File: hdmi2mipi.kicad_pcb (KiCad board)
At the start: 2 copper layers, 60.9 x 56.6 mm, 66 parts, among them J1 USB_C_Receptacle_USB2.0, J4 TP, J5 SWD, J6 BOOT, J7 SWD, Q1 BC846, Q2 BC846, Q3 BC846, Q4 BC846, Q5 BC846, Q6 BC846, U1 SY8079AAC, U3 SY6280AAC, U4 PCA9306DC, U6 W25Q16JVUXIQ, U8 SY6280AAC, X1 SG-210STF, Y1 12MHz

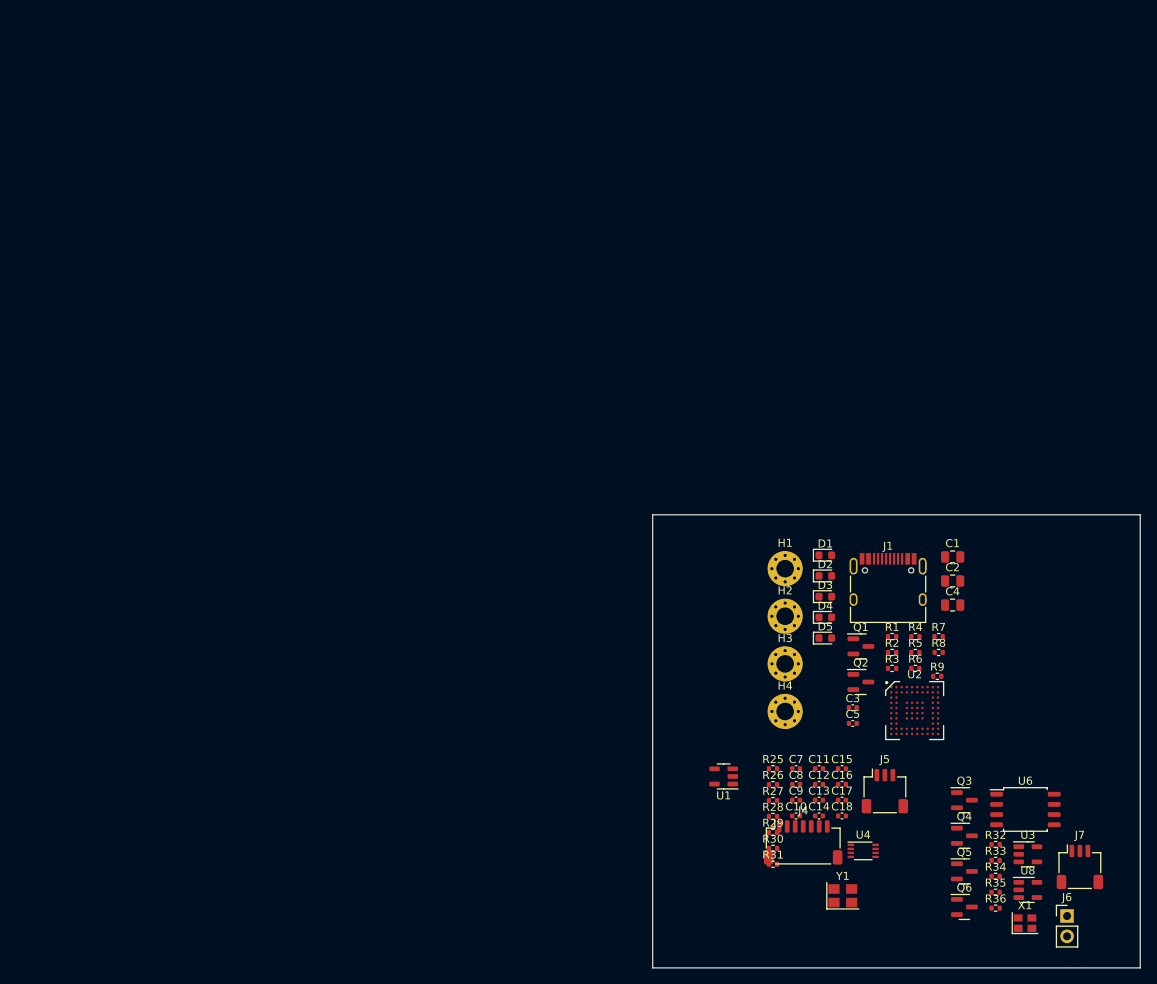
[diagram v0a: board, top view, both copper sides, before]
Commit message: Most of schematic done, experimenting with component placement
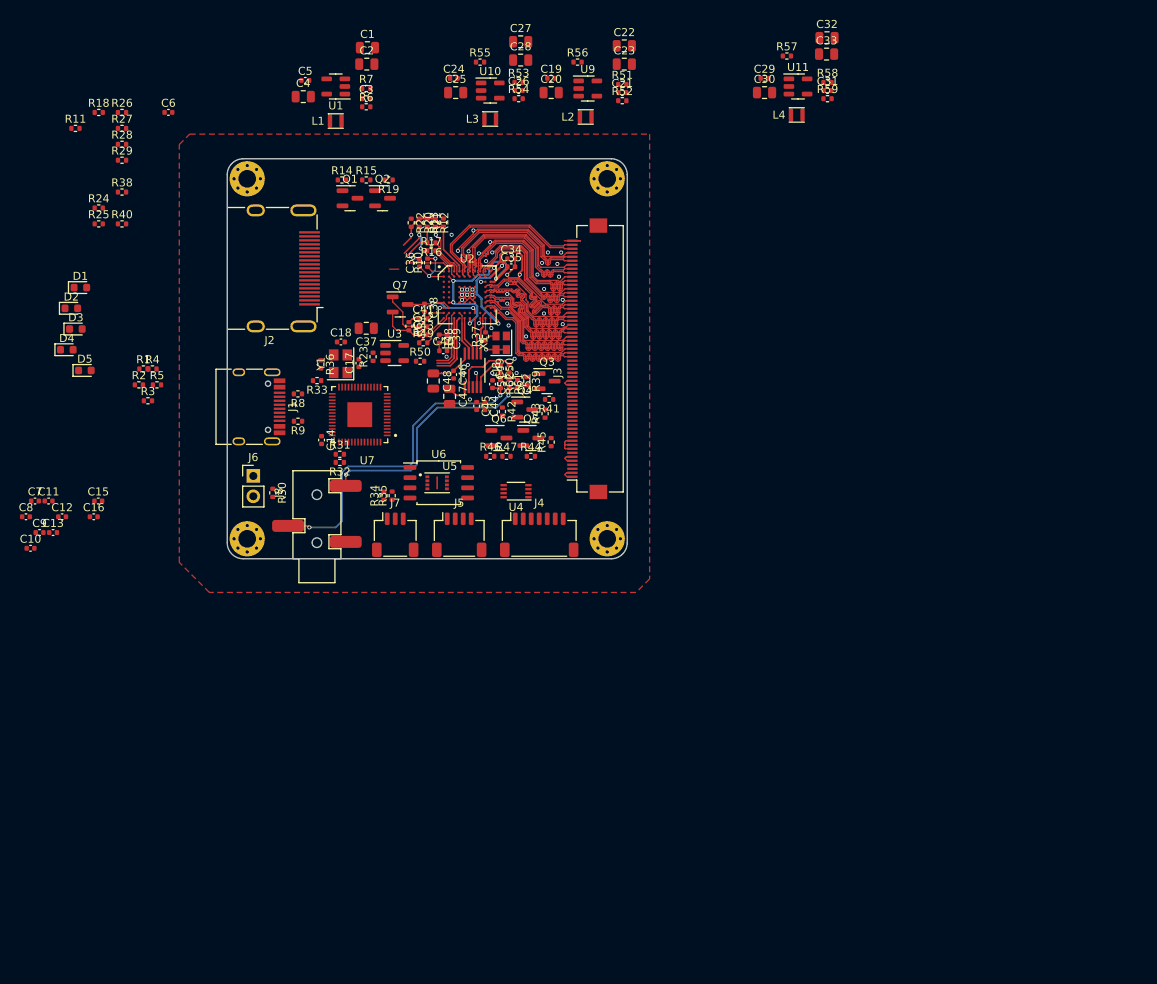
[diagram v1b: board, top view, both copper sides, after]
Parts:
- added C19: 100n, Capacitor_SMD:C_0402_1005Metric, F.Cu at (15.5, -35.1)
- added C20: 22u, Capacitor_SMD:C_0805_2012Metric, F.Cu at (15.5, -33.3)
- added C21: 22p, Capacitor_SMD:C_0402_1005Metric, F.Cu at (24.4, -33.3)
- added C22: 22u, Capacitor_SMD:C_0805_2012Metric, F.Cu at (24.6, -39.1)
- added C23: 22u, Capacitor_SMD:C_0805_2012Metric, F.Cu at (24.6, -36.8)
- added C24: 100n, Capacitor_SMD:C_0402_1005Metric, F.Cu at (3.33, -35.1)
- added C25: 22u, Capacitor_SMD:C_0805_2012Metric, F.Cu at (3.56, -33.3)
- added C26: 22p, Capacitor_SMD:C_0402_1005Metric, F.Cu at (11.4, -33.5)
- added C27: 22u, Capacitor_SMD:C_0805_2012Metric, F.Cu at (11.7, -39.6)
- added C28: 22u, Capacitor_SMD:C_0805_2012Metric, F.Cu at (11.7, -37.3)
- added C29: 100n, Capacitor_SMD:C_0402_1005Metric, F.Cu at (42.2, -35.1)
- added C30: 22u, Capacitor_SMD:C_0805_2012Metric, F.Cu at (42.2, -33.3)
- added C31: 22p, Capacitor_SMD:C_0402_1005Metric, F.Cu at (50.0, -33.5)
- added C32: 22u, Capacitor_SMD:C_0805_2012Metric, F.Cu at (50.0, -40.1)
- added C33: 22u, Capacitor_SMD:C_0805_2012Metric, F.Cu at (49.9, -38.1)
- added C34: 100n, Capacitor_SMD:C_0402_1005Metric, F.Cu at (10.5, -12.5)
- added C35: 100n, Capacitor_SMD:C_0402_1005Metric, F.Cu at (10.5, -11.5)
- added C36: 100n, Capacitor_SMD:C_0402_1005Metric, F.Cu at (-0.97, -12.0)
- added C37: 22u, Capacitor_SMD:C_0805_2012Metric, F.Cu at (-7.62, -3.81)
- added C38: 100n, Capacitor_SMD:C_0402_1005Metric, F.Cu at (-0.34, -6.39)
- added C39: 1n, Capacitor_SMD:C_0402_1005Metric, F.Cu at (2.50, -2.50)
- added C40: 0.1u, Capacitor_SMD:C_0402_1005Metric, F.Cu at (2.00, -1.00)
- added C41: 0.1u, Capacitor_SMD:C_0402_1005Metric, F.Cu at (-0.50, -5.00)
- added C42: 5p, Capacitor_SMD:C_0402_1005Metric, F.Cu at (-0.50, -4.00)
- added C43: 1n, Capacitor_SMD:C_0402_1005Metric, F.Cu at (-0.50, -3.00)
- added C44: 1u, Capacitor_SMD:C_0402_1005Metric, F.Cu at (7.21, 5.92)
- added C45: 100n, Capacitor_SMD:C_0402_1005Metric, F.Cu at (6.18, 5.90)
- added C46: 100n, Capacitor_SMD:C_0402_1005Metric, F.Cu at (3.30, 1.98)
- added C47: 47u, Capacitor_SMD:C_0805_2012Metric, F.Cu at (2.80, 4.70)
- added C48: 47u, Capacitor_SMD:C_0805_2012Metric, F.Cu at (0.76, 2.78)
- added C49: 100n, Capacitor_SMD:C_0402_1005Metric, F.Cu at (10.2, 1.24)
- added C50: 100n, Capacitor_SMD:C_0402_1005Metric, F.Cu at (9.15, 1.23)
- added C51: 39n, Capacitor_SMD:C_0402_1005Metric, F.Cu at (8.16, 3.17)
- added C52: 39n, Capacitor_SMD:C_0402_1005Metric, F.Cu at (11.3, 3.16)
- added C6: ~, Capacitor_SMD:C_0402_1005Metric, F.Cu at (-32.4, -30.8)
- added J2: HDMI_A_1.4, Connector_HDMI:HDMI_A_Molex_208658-1001_Horizontal, F.Cu at (-18.0, -11.3)
- added J3: ~, fpc60:Hirose_FH52-60S-0.5SH_1x60-1MP_P0.50mm_Horizontal, F.Cu at (20.0, 0.00)
- added J8: AudioJack3, custom:Boom-audiojack-PJ-320B, F.Cu at (-13.8, 21.0)
- added L1: 2.2u, custom:Inductor_MSC20FC, F.Cu at (-11.4, -29.7)
- added L2: 2.2u, custom:Inductor_MSC20FC, F.Cu at (19.8, -30.2)
- added L3: 2.2u, custom:Inductor_MSC20FC, F.Cu at (7.87, -30.0)
- added L4: 2.2u, custom:Inductor_MSC20FC, F.Cu at (46.2, -30.5)
- added Q7: 2SC2712, Package_TO_SOT_SMD:SOT-23, F.Cu at (-3.38, -6.79)
- added R10: 2k, Resistor_SMD:R_0402_1005Metric, F.Cu at (0.04, -12.0)
- added R11: 48k, Resistor_SMD:R_0402_1005Metric, F.Cu at (-44.0, -28.8)
- added R12: 0, Resistor_SMD:R_0402_1005Metric, F.Cu at (1.00, -17.0)
- added R13: 1.5k, Resistor_SMD:R_0402_1005Metric, F.Cu at (2.03, -17.0)
- added R14: 4.7k, Resistor_SMD:R_0402_1005Metric, F.Cu at (-10.7, -22.4)
- added R15: 10k, Resistor_SMD:R_0402_1005Metric, F.Cu at (-7.62, -22.4)
- added R16: 33, Resistor_SMD:R_0402_1005Metric, F.Cu at (0.52, -14.5)
- added R17: 33, Resistor_SMD:R_0402_1005Metric, F.Cu at (0.50, -13.5)
- added R18: 1k, Resistor_SMD:R_0402_1005Metric, F.Cu at (-41.1, -30.8)
- added R19: 1k, Resistor_SMD:R_0402_1005Metric, F.Cu at (-4.83, -22.4)
- added R20: 4.7k, Resistor_SMD:R_0402_1005Metric, F.Cu at (-1.00, -17.0)
- added R21: 4.7k, Resistor_SMD:R_0402_1005Metric, F.Cu at (0.00, -17.0)
- added R22: 100k, Resistor_SMD:R_0402_1005Metric, F.Cu at (-2.00, -17.0)
- added R23: 4.7k, Resistor_SMD:R_0402_1005Metric, F.Cu at (-6.77, -0.25)
- added R24: 4.7k, Resistor_SMD:R_0402_1005Metric, F.Cu at (-41.1, -18.9)
- added R37: 33, Resistor_SMD:R_0402_1005Metric, F.Cu at (7.29, -2.79)
- added R38: 10k, Resistor_SMD:R_0402_1005Metric, F.Cu at (-38.1, -20.8)
- added R39: 10k, Resistor_SMD:R_0402_1005Metric, F.Cu at (12.4, 2.79)
- added R40: 10k, Resistor_SMD:R_0402_1005Metric, F.Cu at (-38.1, -16.9)
- added R41: 4.7k, Resistor_SMD:R_0402_1005Metric, F.Cu at (15.2, 5.08)
- added R42: 10k, Resistor_SMD:R_0402_1005Metric, F.Cu at (9.40, 6.60)
- added R43: 4.7k, Resistor_SMD:R_0402_1005Metric, F.Cu at (14.7, 6.86)
- added R44: 10k, Resistor_SMD:R_0402_1005Metric, F.Cu at (13.0, 12.2)
- added R45: 4.7k, Resistor_SMD:R_0402_1005Metric, F.Cu at (15.5, 10.4)
- added R46: 10k, Resistor_SMD:R_0402_1005Metric, F.Cu at (7.87, 12.2)
- added R47: 4.7k, Resistor_SMD:R_0402_1005Metric, F.Cu at (9.91, 12.2)
- added R48: 1k, Resistor_SMD:R_0402_1005Metric, F.Cu at (1.50, -2.50)
- added R49: 1.5k, Resistor_SMD:R_0402_1005Metric, F.Cu at (-0.50, -2.00)
- added R50: 10k, Resistor_SMD:R_0402_1005Metric, F.Cu at (-0.89, 0.31)
- added R51: 10k, Resistor_SMD:R_0402_1005Metric, F.Cu at (24.4, -34.3)
- added R52: 10k, Resistor_SMD:R_0402_1005Metric, F.Cu at (24.4, -32.3)
- added R53: 10k, Resistor_SMD:R_0402_1005Metric, F.Cu at (11.4, -34.5)
- added R54: 8.2k, Resistor_SMD:R_0402_1005Metric, F.Cu at (11.4, -32.5)
- added R55: 10k, Resistor_SMD:R_0402_1005Metric, F.Cu at (6.60, -37.1)
- added R56: 10k, Resistor_SMD:R_0402_1005Metric, F.Cu at (18.8, -37.1)
- added R57: 10k, Resistor_SMD:R_0402_1005Metric, F.Cu at (45.0, -37.8)
- added R58: 10k, Resistor_SMD:R_0402_1005Metric, F.Cu at (50.0, -34.5)
- added R59: 20k, Resistor_SMD:R_0402_1005Metric, F.Cu at (50.0, -32.5)
- added R60: 1k, Resistor_SMD:R_0402_1005Metric, F.Cu at (-2.29, -4.06)
- added R61: 330, Resistor_SMD:R_0402_1005Metric, F.Cu at (10.2, 3.15)
- added R62: 330, Resistor_SMD:R_0402_1005Metric, F.Cu at (9.17, 3.15)
- added U10: SY8079AAC, Package_TO_SOT_SMD:SOT-23-5, F.Cu at (7.87, -33.5)
- added U11: SY8079AAC, Package_TO_SOT_SMD:SOT-23-5, F.Cu at (46.3, -34.0)
- added U5: W25Q16JVUXIQ, custom:PSON50P300X200X60-9N, F.Cu at (1.24, 15.5)
- added U7: RP2040, custom:QFN40P700X700X90-57N, F.Cu at (-8.44, 6.98)
- added U9: SY8079AAC, Package_TO_SOT_SMD:SOT-23-5, F.Cu at (20.1, -33.8)
- J5: value SWD -> QWIIC; footprint Connector_JST:JST_SH_SM03B-SRSS-TB_1x03-1MP_P1.00mm_Horizontal -> Connector_JST:JST_SH_SM04B-SRSS-TB_1x04-1MP_P1.00mm_Horizontal
- R25, R28: value 1k -> 4.7k
- R26, R27: value 27 -> 4.7k
- R29: value 100 -> 4.7k
- U8: value SY6280AAC -> MS4344; footprint Package_TO_SOT_SMD:SOT-23-5 -> custom:SOP50P490X110-10N
- moved R26 117.0 mm to (-38.1, -30.8)
- moved R27 117.0 mm to (-38.1, -28.8)
- moved R28 117.0 mm to (-38.1, -26.8)
- moved R29 117.0 mm to (-38.1, -24.8)
- moved J6 115.6 mm to (-21.7, 14.7)
- moved R25 108.4 mm to (-41.1, -16.9)
- moved R36 108.3 mm to (-13.3, 0.70), turned to -90 degrees
- moved C5 105.6 mm to (-15.2, -34.8)
- moved R33 103.9 mm to (-13.8, 2.73), turned to 180 degrees
- moved C4 103.1 mm to (-15.5, -32.8)
- moved C11 102.0 mm to (-47.3, 17.8)
- moved C8 101.9 mm to (-50.2, 19.8)
- moved C13 101.4 mm to (-46.8, 21.7)
- moved C10 101.4 mm to (-49.6, 23.7)
- moved R4 101.1 mm to (-34.3, 1.27)
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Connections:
- net MC_VSUPPLY_11 renamed +1V1
- net MC_VSUPPLY_12 renamed +1V2
- net VIN renamed VBUS
- J4 pad 5: /TP_VSUPPLY_18 -> +1V8
- J4 pad 6: /TP_VSUPPLY_33 -> 3V3_HDMI
- J5 pad 1: Net-(J5-Pin_1) -> GND
- J5 pad 2: GND -> +3V3
- J5 pad MP: (no net) -> GND
- Q3 pad 1: Net-(Q3-B) -> 3V3_S2
- Q4 pad 1: Net-(Q4-B) -> 3V3_S1
- Q5 pad 1: Net-(Q5-B) -> 1V8_S2
- Q6 pad 1: Net-(Q6-B) -> 1V8_S1
- R1 pad 1: unconnected-(R1-Pad1) -> Net-(U7-GPIO11)
- R2 pad 1: unconnected-(R2-Pad1) -> Net-(U7-GPIO12)
- R25 pad 1: /Microcontroller/RP_QSPI_CSN -> +1V8
- R25 pad 2: /Microcontroller/RP_BTN -> Net-(J4-Pin_4)
- R26 pad 1: /Microcontroller/USB_DN -> +3V3
- R26 pad 2: Net-(U5-USB_DM) -> Net-(J5-Pin_3)
- R27 pad 1: Net-(U5-USB_DP) -> 3V3_HDMI
- R27 pad 2: /Microcontroller/USB_DP -> Net-(U2-I2C_SCL)
- R28 pad 1: Net-(U5-RUN) -> +3V3
- R28 pad 2: +3V3 -> Net-(J5-Pin_4)
- R29 pad 1: Net-(J5-Pin_1) -> 3V3_HDMI
- R29 pad 2: Net-(U5-SWCLK) -> Net-(U2-I2C_SDA)
- R3 pad 1: unconnected-(R3-Pad1) -> Net-(U7-GPIO13)
- R4 pad 1: unconnected-(R4-Pad1) -> Net-(U7-GPIO14)
- R5 pad 1: unconnected-(R5-Pad1) -> Net-(U7-GPIO10)
- U2 pad A5: Net-(J3-Pin_3) -> /DSI1_D3_P
- U2 pad A6: Net-(J3-Pin_6) -> /DSI1_D2_P
- U2 pad A7: Net-(J3-Pin_9) -> /DSI1_C_P
- U2 pad A8: Net-(J3-Pin_12) -> /DSI1_D1_P
- U2 pad A9: Net-(J3-Pin_15) -> /DSI1_D0_P
- U2 pad B1: VDD33_HDMI -> 3V3_HDMI
- U2 pad B5: Net-(J3-Pin_2) -> /DSI1_D3_N
- U2 pad B6: Net-(J3-Pin_5) -> /DSI1_D2_N
- U2 pad B7: Net-(J3-Pin_8) -> /DSI1_C_N
- U2 pad B8: Net-(J3-Pin_11) -> /DSI1_D1_N
- U2 pad B9: Net-(J3-Pin_14) -> /DSI1_D0_N
- U2 pad C1: Net-(J2-CK+) -> /HDMI_C_P
- U2 pad C2: Net-(J2-CK-) -> /HDMI_C_N
- U2 pad D1: Net-(J2-D0+) -> /HDMI_0_P
- U2 pad D10: Net-(J3-Pin_18) -> /DSI0_D3_P
- U2 pad D2: Net-(J2-D0-) -> /HDMI_0_N
- U2 pad D9: Net-(J3-Pin_17) -> /DSI0_D3_N
- U2 pad E1: Net-(J2-D1+) -> /HDMI_1_P
- U2 pad E10: Net-(J3-Pin_21) -> /DSI0_D2_P
- U2 pad E2: Net-(J2-D1-) -> /HDMI_1_N
- U2 pad E9: Net-(J3-Pin_20) -> /DSI0_D2_N
- U2 pad F1: Net-(J2-D2+) -> /HDMI_2_P
- U2 pad F10: Net-(J3-Pin_24) -> /DSI0_C_P
- U2 pad F2: Net-(J2-D2-) -> /HDMI_2_N
- U2 pad F9: Net-(J3-Pin_23) -> /DSI0_C_N
- U2 pad G1: VDD33_HDMI -> 3V3_HDMI
- U2 pad G10: Net-(J3-Pin_27) -> /DSI0_D1_P
- U2 pad G9: Net-(J3-Pin_26) -> /DSI0_D1_N
- U2 pad H10: Net-(J3-Pin_30) -> /DSI0_D0_P
- U2 pad H2: VDD33_HDMI -> 3V3_HDMI
- U2 pad H9: Net-(J3-Pin_29) -> /DSI0_D0_N
- U2 pad J1: unconnected-(U2-BIASDA-PadJ1) -> Net-(U2-BIASDA)
- U2 pad J2: unconnected-(U2-DAOUT-PadJ2) -> Net-(U2-DAOUT)
- U2 pad J3: MC_I2C_INT -> Net-(U2-INT)
- U2 pad J4: unconnected-(U2-A_OSCK-PadJ4) -> Net-(U2-A_OSCK)
- U2 pad J7: VDD33_HDMI -> 3V3_HDMI
- U2 pad J9: unconnected-(U2-A_SD0-PadJ9) -> Net-(U2-A_SD0)
- U2 pad K1: unconnected-(U2-PCKIN-PadK1) -> Net-(U2-PCKIN)
- U2 pad K2: unconnected-(U2-PFIL-PadK2) -> Net-(U2-PFIL)
- U2 pad K5: unconnected-(U2-A_WFS-PadK5) -> Net-(U2-A_WFS)
- U2 pad K7: unconnected-(U2-A_SCK-PadK7) -> Net-(U2-A_SCK)
- U2 pad K8: MC_I2C_RESET -> Net-(U2-~{RESET})
- U3 pad 1: VDD33_HDMI -> 3V3_HDMI
- U4 pad 2: /TP_VSUPPLY_18 -> +1V8
- U8 pad 1: Net-(J3-Pin_36) -> Net-(U2-A_SD0)
- U8 pad 2: GND -> Net-(U2-A_SCK)
- U8 pad 3: Net-(U8-SET) -> Net-(U2-A_WFS)
- U8 pad 4: Net-(U7-GPIO3) -> Net-(U2-A_OSCK)
- U8 pad 5: +3V3 -> Net-(U8-VQ)
- X1 pad 1: VDD33_HDMI -> 3V3_HDMI
- X1 pad 4: VDD33_HDMI -> 3V3_HDMI
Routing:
- net GND: track 0.00 -> 157.8 mm, vias 0 -> 45
- net /AUDIO_R: track 0.00 -> 42.0 mm, vias 0 -> 2
- net /AUDIO_L: track 0.00 -> 30.5 mm, vias 0 -> 2
- net +1V1: track 0.00 -> 24.3 mm, vias 0 -> 4
- net 3V3_HDMI: track 0.00 -> 23.5 mm, vias 0 -> 5
- net /DSI0_D1_N: track 0.00 -> 22.8 mm
- net /DSI1_D3_N: track 0.00 -> 22.2 mm
- net /DSI1_D3_P: track 0.00 -> 22.2 mm
- net /DSI1_D2_N: track 0.00 -> 22.0 mm
- net /DSI1_C_N: track 0.00 -> 21.9 mm
- net /DSI1_D1_N: track 0.00 -> 21.9 mm
- net /DSI1_D2_P: track 0.00 -> 21.9 mm
- net /DSI1_C_P: track 0.00 -> 21.9 mm
- net /DSI1_D1_P: track 0.00 -> 21.9 mm
- net /DSI0_D1_P: track 0.00 -> 21.8 mm
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- added copper zone on In2.Cu, net +1V1
- added copper zone on In2.Cu, net +1V2
- added copper zone on In2.Cu, net +3V3
- added copper zone on F.Cu, net GND
- added copper zone on In1.Cu, net GND
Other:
- board size 60.9 x 56.6 mm -> 50 x 50 mm
- copper layers 2 -> 4
